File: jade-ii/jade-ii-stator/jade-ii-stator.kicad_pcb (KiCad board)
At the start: 2 copper layers, 93 x 127.3 mm, 0 parts

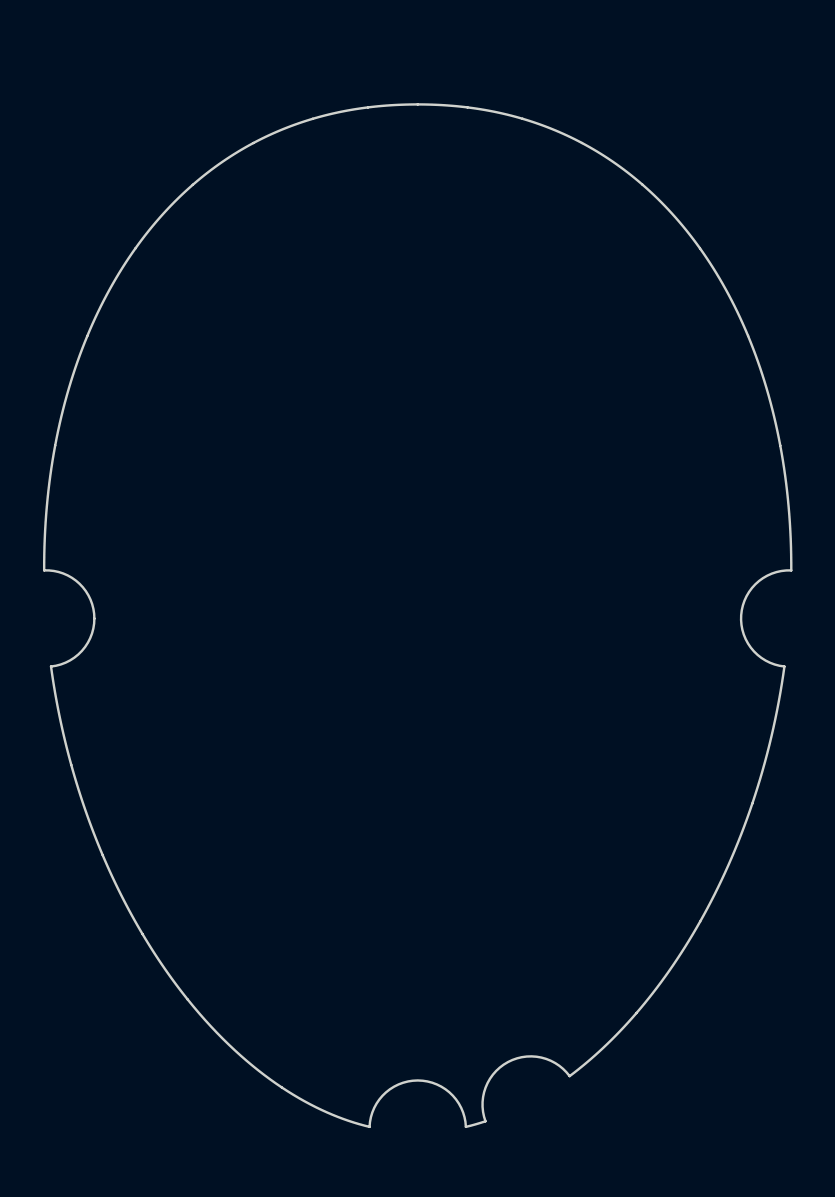
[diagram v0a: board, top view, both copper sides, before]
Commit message: jade: finished stator
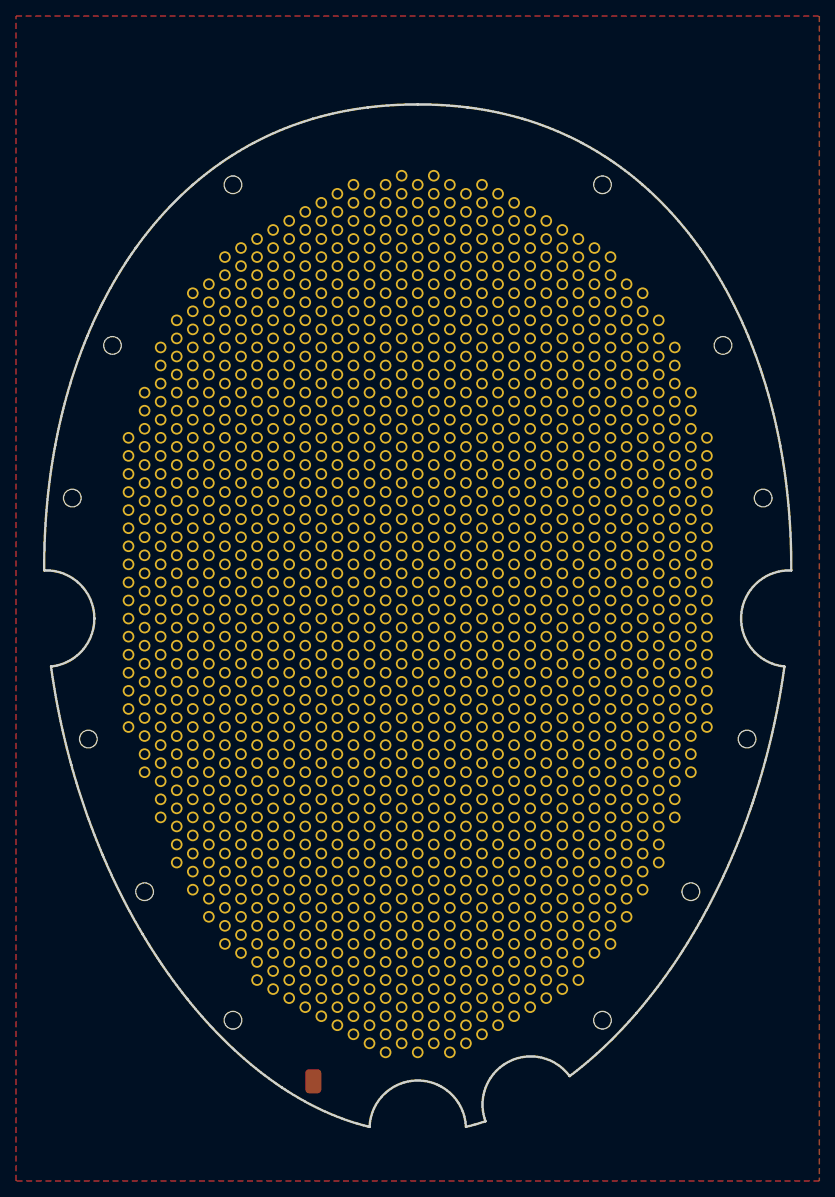
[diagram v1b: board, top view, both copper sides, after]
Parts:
- added H1: MountingHole_Pad, MountingHole:MountingHole_2.2mm_M2_Pad, F.Cu at (26.0, -12.4)
- added H1: MountingHole_Pad, MountingHole:MountingHole_2.2mm_M2_Pad, F.Cu at (-2.00, 12.4)
- added H1: MountingHole_Pad, MountingHole:MountingHole_2.2mm_M2_Pad, F.Cu at (8.00, -31.5)
- added H1: MountingHole_Pad, MountingHole:MountingHole_2.2mm_M2_Pad, F.Cu at (-28.0, 15.8)
- added H1: MountingHole_Pad, MountingHole:MountingHole_2.2mm_M2_Pad, F.Cu at (-10.0, -50.6)
- added H1: MountingHole_Pad, MountingHole:MountingHole_2.2mm_M2_Pad, F.Cu at (-16.0, -24.8)
- added H1: MountingHole_Pad, MountingHole:MountingHole_2.2mm_M2_Pad, F.Cu at (-4.00, 20.2)
- added H1: MountingHole_Pad, MountingHole:MountingHole_2.2mm_M2_Pad, F.Cu at (18.0, -21.4)
- added H1: MountingHole_Pad, MountingHole:MountingHole_2.2mm_M2_Pad, F.Cu at (0.00, 36.0)
- added H1: MountingHole_Pad, MountingHole:MountingHole_2.2mm_M2_Pad, F.Cu at (8.00, 0.00)
- added H1: MountingHole_Pad, MountingHole:MountingHole_2.2mm_M2_Pad, F.Cu at (22.0, 5.62)
- added H1: MountingHole_Pad, MountingHole:MountingHole_2.2mm_M2_Pad, F.Cu at (12.0, -27.0)
- added H1: MountingHole_Pad, MountingHole:MountingHole_2.2mm_M2_Pad, F.Cu at (12.0, -31.5)
- added H1: MountingHole_Pad, MountingHole:MountingHole_2.2mm_M2_Pad, F.Cu at (-4.00, 0.00)
- added H1: MountingHole_Pad, MountingHole:MountingHole_2.2mm_M2_Pad, F.Cu at (-20.0, 9.00)
- added H1: MountingHole_Pad, MountingHole:MountingHole_2.2mm_M2_Pad, F.Cu at (-12.0, 47.2)
- added H1: MountingHole_Pad, MountingHole:MountingHole_2.2mm_M2_Pad, F.Cu at (16.0, -31.5)
- added H1: MountingHole_Pad, MountingHole:MountingHole_2.2mm_M2_Pad, F.Cu at (20.0, -36.0)
- added H1: MountingHole_Pad, MountingHole:MountingHole_2.2mm_M2_Pad, F.Cu at (-2.00, 43.9)
- added H1: MountingHole_Pad, MountingHole:MountingHole_2.2mm_M2_Pad, F.Cu at (4.00, -51.8)
- added H1: MountingHole_Pad, MountingHole:MountingHole_2.2mm_M2_Pad, F.Cu at (26.0, 5.62)
- added H1: MountingHole_Pad, MountingHole:MountingHole_2.2mm_M2_Pad, F.Cu at (-18.0, -1.12)
- added H1: MountingHole_Pad, MountingHole:MountingHole_2.2mm_M2_Pad, F.Cu at (8.00, 49.5)
- added H1: MountingHole_Pad, MountingHole:MountingHole_2.2mm_M2_Pad, F.Cu at (26.0, -41.6)
- added H1: MountingHole_Pad, MountingHole:MountingHole_2.2mm_M2_Pad, F.Cu at (-14.0, 46.1)
- added H1: MountingHole_Pad, MountingHole:MountingHole_2.2mm_M2_Pad, F.Cu at (22.0, 21.4)
- added H1: MountingHole_Pad, MountingHole:MountingHole_2.2mm_M2_Pad, F.Cu at (-16.0, 2.25)
- added H1: MountingHole_Pad, MountingHole:MountingHole_2.2mm_M2_Pad, F.Cu at (26.0, 30.4)
- added H1: MountingHole_Pad, MountingHole:MountingHole_2.2mm_M2_Pad, F.Cu at (-28.0, -33.8)
- added H1: MountingHole_Pad, MountingHole:MountingHole_2.2mm_M2_Pad, F.Cu at (0.00, 51.8)
- added H1: MountingHole_Pad, MountingHole:MountingHole_2.2mm_M2_Pad, F.Cu at (20.0, 18.0)
- added H1: MountingHole_Pad, MountingHole:MountingHole_2.2mm_M2_Pad, F.Cu at (-2.00, 37.1)
- added H1: MountingHole_Pad, MountingHole:MountingHole_2.2mm_M2_Pad, F.Cu at (-10.0, -52.9)
- added H1: MountingHole_Pad, MountingHole:MountingHole_2.2mm_M2_Pad, F.Cu at (-2.00, 41.6)
- added H1: MountingHole_Pad, MountingHole:MountingHole_2.2mm_M2_Pad, F.Cu at (18.0, -10.1)
- added H1: MountingHole_Pad, MountingHole:MountingHole_2.2mm_M2_Pad, F.Cu at (-34.0, 1.12)
- added H1: MountingHole_Pad, MountingHole:MountingHole_2.2mm_M2_Pad, F.Cu at (26.0, 19.1)
- added H1: MountingHole_Pad, MountingHole:MountingHole_2.2mm_M2_Pad, F.Cu at (0.00, 22.5)
- added H1: MountingHole_Pad, MountingHole:MountingHole_2.2mm_M2_Pad, F.Cu at (-18.0, 12.4)
- added H1: MountingHole_Pad, MountingHole:MountingHole_2.2mm_M2_Pad, F.Cu at (-18.0, -21.4)
- added H1: MountingHole_Pad, MountingHole:MountingHole_2.2mm_M2_Pad, F.Cu at (-26.0, 1.12)
- added H1: MountingHole_Pad, MountingHole:MountingHole_2.2mm_M2_Pad, F.Cu at (-2.00, -34.9)
- added H1: MountingHole_Pad, MountingHole:MountingHole_2.2mm_M2_Pad, F.Cu at (14.0, -30.4)
- added H1: MountingHole_Pad, MountingHole:MountingHole_2.2mm_M2_Pad, F.Cu at (-16.0, 22.5)
- added H1: MountingHole_Pad, MountingHole:MountingHole_2.2mm_M2_Pad, F.Cu at (-6.00, 10.1)
- added H1: MountingHole_Pad, MountingHole:MountingHole_2.2mm_M2_Pad, F.Cu at (28.0, 33.8)
- added H1: MountingHole_Pad, MountingHole:MountingHole_2.2mm_M2_Pad, F.Cu at (-32.0, 6.75)
- added H1: MountingHole_Pad, MountingHole:MountingHole_2.2mm_M2_Pad, F.Cu at (-6.00, 19.1)
- added H1: MountingHole_Pad, MountingHole:MountingHole_2.2mm_M2_Pad, F.Cu at (-8.00, -29.2)
- added H1: MountingHole_Pad, MountingHole:MountingHole_2.2mm_M2_Pad, F.Cu at (-18.0, 28.1)
- added H1: MountingHole_Pad, MountingHole:MountingHole_2.2mm_M2_Pad, F.Cu at (30.0, -32.6)
- added H1: MountingHole_Pad, MountingHole:MountingHole_2.2mm_M2_Pad, F.Cu at (0.00, 47.2)
- added H1: MountingHole_Pad, MountingHole:MountingHole_2.2mm_M2_Pad, F.Cu at (8.00, -9.00)
- added H1: MountingHole_Pad, MountingHole:MountingHole_2.2mm_M2_Pad, F.Cu at (6.00, 37.1)
- added H1: MountingHole_Pad, MountingHole:MountingHole_2.2mm_M2_Pad, F.Cu at (-4.00, -20.2)
- added H1: MountingHole_Pad, MountingHole:MountingHole_2.2mm_M2_Pad, F.Cu at (28.0, -20.2)
- added H1: MountingHole_Pad, MountingHole:MountingHole_2.2mm_M2_Pad, F.Cu at (16.0, 42.8)
- added H1: MountingHole_Pad, MountingHole:MountingHole_2.2mm_M2_Pad, F.Cu at (22.0, -5.62)
- added H1: MountingHole_Pad, MountingHole:MountingHole_2.2mm_M2_Pad, F.Cu at (16.0, -13.5)
- added H1: MountingHole_Pad, MountingHole:MountingHole_2.2mm_M2_Pad, F.Cu at (-8.00, 27.0)
- added H1: MountingHole_Pad, MountingHole:MountingHole_2.2mm_M2_Pad, F.Cu at (2.00, 48.4)
- added H1: MountingHole_Pad, MountingHole:MountingHole_2.2mm_M2_Pad, F.Cu at (-22.0, -10.1)
- added H1: MountingHole_Pad, MountingHole:MountingHole_2.2mm_M2_Pad, F.Cu at (4.00, -13.5)
- added H1: MountingHole_Pad, MountingHole:MountingHole_2.2mm_M2_Pad, F.Cu at (4.00, 42.8)
- added H1: MountingHole_Pad, MountingHole:MountingHole_2.2mm_M2_Pad, F.Cu at (20.0, -45.0)
- added H1: MountingHole_Pad, MountingHole:MountingHole_2.2mm_M2_Pad, F.Cu at (-22.0, -34.9)
- added H1: MountingHole_Pad, MountingHole:MountingHole_2.2mm_M2_Pad, F.Cu at (0.00, -33.8)
- added H1: MountingHole_Pad, MountingHole:MountingHole_2.2mm_M2_Pad, F.Cu at (30.0, 7.88)
- added H1: MountingHole_Pad, MountingHole:MountingHole_2.2mm_M2_Pad, F.Cu at (12.0, 40.5)
- added H1: MountingHole_Pad, MountingHole:MountingHole_2.2mm_M2_Pad, F.Cu at (-36.0, 4.50)
- added H1: MountingHole_Pad, MountingHole:MountingHole_2.2mm_M2_Pad, F.Cu at (-2.00, -52.9)
- added H1: MountingHole_Pad, MountingHole:MountingHole_2.2mm_M2_Pad, F.Cu at (4.00, -42.8)
- added H1: MountingHole_Pad, MountingHole:MountingHole_2.2mm_M2_Pad, F.Cu at (-32.0, 11.2)
- added H1: MountingHole_Pad, MountingHole:MountingHole_2.2mm_M2_Pad, F.Cu at (-34.0, 12.4)
- added H1: MountingHole_Pad, MountingHole:MountingHole_2.2mm_M2_Pad, F.Cu at (16.0, 2.25)
- added H1: MountingHole_Pad, MountingHole:MountingHole_2.2mm_M2_Pad, F.Cu at (-22.0, 25.9)
- added H1: MountingHole_Pad, MountingHole:MountingHole_2.2mm_M2_Pad, F.Cu at (22.0, -43.9)
- added H1: MountingHole_Pad, MountingHole:MountingHole_2.2mm_M2_Pad, F.Cu at (28.0, -29.2)
- added H1: MountingHole_Pad, MountingHole:MountingHole_2.2mm_M2_Pad, F.Cu at (-4.00, -6.75)
- added H1: MountingHole_Pad, MountingHole:MountingHole_2.2mm_M2_Pad, F.Cu at (16.0, -45.0)
- added H1: MountingHole_Pad, MountingHole:MountingHole_2.2mm_M2_Pad, F.Cu at (10.0, -5.62)
- added H1: MountingHole_Pad, MountingHole:MountingHole_2.2mm_M2_Pad, F.Cu at (2.00, -10.1)
- added H1: MountingHole_Pad, MountingHole:MountingHole_2.2mm_M2_Pad, F.Cu at (-18.0, 32.6)
- added H1: MountingHole_Pad, MountingHole:MountingHole_2.2mm_M2_Pad, F.Cu at (6.00, -50.6)
- added H1: MountingHole_Pad, MountingHole:MountingHole_2.2mm_M2_Pad, F.Cu at (-32.0, -13.5)
- added H1: MountingHole_Pad, MountingHole:MountingHole_2.2mm_M2_Pad, F.Cu at (-26.0, 30.4)
- added H1: MountingHole_Pad, MountingHole:MountingHole_2.2mm_M2_Pad, F.Cu at (-10.0, 39.4)
- added H1: MountingHole_Pad, MountingHole:MountingHole_2.2mm_M2_Pad, F.Cu at (-36.0, 2.25)
- added H1: MountingHole_Pad, MountingHole:MountingHole_2.2mm_M2_Pad, F.Cu at (6.00, 39.4)
- added H1: MountingHole_Pad, MountingHole:MountingHole_2.2mm_M2_Pad, F.Cu at (-6.00, -16.9)
- added H1: MountingHole_Pad, MountingHole:MountingHole_2.2mm_M2_Pad, F.Cu at (34.0, 5.62)
- added H1: MountingHole_Pad, MountingHole:MountingHole_2.2mm_M2_Pad, F.Cu at (-8.00, -20.2)
- added H1: MountingHole_Pad, MountingHole:MountingHole_2.2mm_M2_Pad, F.Cu at (-12.0, -20.2)
- added H1: MountingHole_Pad, MountingHole:MountingHole_2.2mm_M2_Pad, F.Cu at (-14.0, 16.9)
- added H1: MountingHole_Pad, MountingHole:MountingHole_2.2mm_M2_Pad, F.Cu at (28.0, -36.0)
- added H1: MountingHole_Pad, MountingHole:MountingHole_2.2mm_M2_Pad, F.Cu at (-6.00, -3.38)
- added H1: MountingHole_Pad, MountingHole:MountingHole_2.2mm_M2_Pad, F.Cu at (8.00, 13.5)
- added H1: MountingHole_Pad, MountingHole:MountingHole_2.2mm_M2_Pad, F.Cu at (10.0, 25.9)
- added H1: MountingHole_Pad, MountingHole:MountingHole_2.2mm_M2_Pad, F.Cu at (-2.00, -10.1)
- added H1: MountingHole_Pad, MountingHole:MountingHole_2.2mm_M2_Pad, F.Cu at (22.0, 39.4)
- added H1: MountingHole_Pad, MountingHole:MountingHole_2.2mm_M2_Pad, F.Cu at (14.0, -21.4)
- added H1: MountingHole_Pad, MountingHole:MountingHole_2.2mm_M2_Pad, F.Cu at (-12.0, -29.2)
- added H1: MountingHole_Pad, MountingHole:MountingHole_2.2mm_M2_Pad, F.Cu at (4.00, -2.25)
- added H1: MountingHole_Pad, MountingHole:MountingHole_2.2mm_M2_Pad, F.Cu at (-8.00, -4.50)
- added H1: MountingHole_Pad, MountingHole:MountingHole_2.2mm_M2_Pad, F.Cu at (-8.00, -54.0)
- added H1: MountingHole_Pad, MountingHole:MountingHole_2.2mm_M2_Pad, F.Cu at (4.00, 2.25)
- added H1: MountingHole_Pad, MountingHole:MountingHole_2.2mm_M2_Pad, F.Cu at (32.0, -13.5)
- added H1: MountingHole_Pad, MountingHole:MountingHole_2.2mm_M2_Pad, F.Cu at (14.0, 28.1)
- added H1: MountingHole_Pad, MountingHole:MountingHole_2.2mm_M2_Pad, F.Cu at (2.00, -23.6)
- added H1: MountingHole_Pad, MountingHole:MountingHole_2.2mm_M2_Pad, F.Cu at (-22.0, -32.6)
- added H1: MountingHole_Pad, MountingHole:MountingHole_2.2mm_M2_Pad, F.Cu at (14.0, 30.4)
- added H1: MountingHole_Pad, MountingHole:MountingHole_2.2mm_M2_Pad, F.Cu at (14.0, 7.88)
- added H1: MountingHole_Pad, MountingHole:MountingHole_2.2mm_M2_Pad, F.Cu at (-16.0, -6.75)
- added H1: MountingHole_Pad, MountingHole:MountingHole_2.2mm_M2_Pad, F.Cu at (14.0, 21.4)
- added H1: MountingHole_Pad, MountingHole:MountingHole_2.2mm_M2_Pad, F.Cu at (4.00, 24.8)
- added H1: MountingHole_Pad, MountingHole:MountingHole_2.2mm_M2_Pad, F.Cu at (30.0, -14.6)
- added H1: MountingHole_Pad, MountingHole:MountingHole_2.2mm_M2_Pad, F.Cu at (-4.00, 24.8)
- added H1: MountingHole_Pad, MountingHole:MountingHole_2.2mm_M2_Pad, F.Cu at (14.0, 46.1)
- added H1: MountingHole_Pad, MountingHole:MountingHole_2.2mm_M2_Pad, F.Cu at (-20.0, -2.25)
- added H1: MountingHole_Pad, MountingHole:MountingHole_2.2mm_M2_Pad, F.Cu at (-22.0, 39.4)
- added H1: MountingHole_Pad, MountingHole:MountingHole_2.2mm_M2_Pad, F.Cu at (-10.0, 50.6)
- added H1: MountingHole_Pad, MountingHole:MountingHole_2.2mm_M2_Pad, F.Cu at (0.00, 11.2)
- added H1: MountingHole_Pad, MountingHole:MountingHole_2.2mm_M2_Pad, F.Cu at (28.0, 15.8)
- added H1: MountingHole_Pad, MountingHole:MountingHole_2.2mm_M2_Pad, F.Cu at (-4.00, 4.50)
- added H1: MountingHole_Pad, MountingHole:MountingHole_2.2mm_M2_Pad, F.Cu at (20.0, 38.2)
- added H1: MountingHole_Pad, MountingHole:MountingHole_2.2mm_M2_Pad, F.Cu at (-16.0, -18.0)
- added H1: MountingHole_Pad, MountingHole:MountingHole_2.2mm_M2_Pad, F.Cu at (18.0, -32.6)
- added H1: MountingHole_Pad, MountingHole:MountingHole_2.2mm_M2_Pad, F.Cu at (32.0, -15.8)
- added H1: MountingHole_Pad, MountingHole:MountingHole_2.2mm_M2_Pad, F.Cu at (-20.0, 33.8)
- added H1: MountingHole_Pad, MountingHole:MountingHole_2.2mm_M2_Pad, F.Cu at (20.0, 13.5)
- added H1: MountingHole_Pad, MountingHole:MountingHole_2.2mm_M2_Pad, F.Cu at (34.0, 12.4)
- added H1: MountingHole_Pad, MountingHole:MountingHole_2.2mm_M2_Pad, F.Cu at (20.0, 0.00)
- added H1: MountingHole_Pad, MountingHole:MountingHole_2.2mm_M2_Pad, F.Cu at (-26.0, 5.62)
- added H1: MountingHole_Pad, MountingHole:MountingHole_2.2mm_M2_Pad, F.Cu at (-4.00, -33.8)
- added H1: MountingHole_Pad, MountingHole:MountingHole_2.2mm_M2_Pad, F.Cu at (-4.00, -36.0)
- added H1: MountingHole_Pad, MountingHole:MountingHole_2.2mm_M2_Pad, F.Cu at (22.0, -41.6)
- added H1: MountingHole_Pad, MountingHole:MountingHole_2.2mm_M2_Pad, F.Cu at (26.0, 32.6)
- added H1: MountingHole_Pad, MountingHole:MountingHole_2.2mm_M2_Pad, F.Cu at (-24.0, 11.2)
- added H1: MountingHole_Pad, MountingHole:MountingHole_2.2mm_M2_Pad, F.Cu at (4.00, 13.5)
- added H1: MountingHole_Pad, MountingHole:MountingHole_2.2mm_M2_Pad, F.Cu at (30.0, -5.62)
- added H1: MountingHole_Pad, MountingHole:MountingHole_2.2mm_M2_Pad, F.Cu at (4.00, 22.5)
- added H1: MountingHole_Pad, MountingHole:MountingHole_2.2mm_M2_Pad, F.Cu at (-12.0, -49.5)
- added H1: MountingHole_Pad, MountingHole:MountingHole_2.2mm_M2_Pad, F.Cu at (2.00, -39.4)
- added H1: MountingHole_Pad, MountingHole:MountingHole_2.2mm_M2_Pad, F.Cu at (-6.00, -48.4)
- added H1: MountingHole_Pad, MountingHole:MountingHole_2.2mm_M2_Pad, F.Cu at (-26.0, -3.38)
- added H1: MountingHole_Pad, MountingHole:MountingHole_2.2mm_M2_Pad, F.Cu at (-32.0, -6.75)
- added H1: MountingHole_Pad, MountingHole:MountingHole_2.2mm_M2_Pad, F.Cu at (0.00, 33.8)
- added H1: MountingHole_Pad, MountingHole:MountingHole_2.2mm_M2_Pad, F.Cu at (-4.00, -42.8)
- added H1: MountingHole_Pad, MountingHole:MountingHole_2.2mm_M2_Pad, F.Cu at (12.0, -36.0)
- added H1: MountingHole_Pad, MountingHole:MountingHole_2.2mm_M2_Pad, F.Cu at (-10.0, 23.6)
- added H1: MountingHole_Pad, MountingHole:MountingHole_2.2mm_M2_Pad, F.Cu at (16.0, 33.8)
- added H1: MountingHole_Pad, MountingHole:MountingHole_2.2mm_M2_Pad, F.Cu at (-14.0, -3.38)
- added H1: MountingHole_Pad, MountingHole:MountingHole_2.2mm_M2_Pad, F.Cu at (20.0, 15.8)
- added H1: MountingHole_Pad, MountingHole:MountingHole_2.2mm_M2_Pad, F.Cu at (-18.0, 34.9)
- added H1: MountingHole_Pad, MountingHole:MountingHole_2.2mm_M2_Pad, F.Cu at (-32.0, 2.25)
- added H1: MountingHole_Pad, MountingHole:MountingHole_2.2mm_M2_Pad, F.Cu at (-26.0, -5.62)
- added H1: MountingHole_Pad, MountingHole:MountingHole_2.2mm_M2_Pad, F.Cu at (-10.0, -3.38)
- added H1: MountingHole_Pad, MountingHole:MountingHole_2.2mm_M2_Pad, F.Cu at (-4.00, -9.00)
- added H1: MountingHole_Pad, MountingHole:MountingHole_2.2mm_M2_Pad, F.Cu at (-6.00, 41.6)
- added H1: MountingHole_Pad, MountingHole:MountingHole_2.2mm_M2_Pad, F.Cu at (28.0, 0.00)
- added H1: MountingHole_Pad, MountingHole:MountingHole_2.2mm_M2_Pad, F.Cu at (4.00, 4.50)
- added H1: MountingHole_Pad, MountingHole:MountingHole_2.2mm_M2_Pad, F.Cu at (18.0, -48.4)
- added H1: MountingHole_Pad, MountingHole:MountingHole_2.2mm_M2_Pad, F.Cu at (-20.0, -11.2)
- added H1: MountingHole_Pad, MountingHole:MountingHole_2.2mm_M2_Pad, F.Cu at (-32.0, 4.50)
- added H1: MountingHole_Pad, MountingHole:MountingHole_2.2mm_M2_Pad, F.Cu at (-16.0, -13.5)
- added H1: MountingHole_Pad, MountingHole:MountingHole_2.2mm_M2_Pad, F.Cu at (10.0, 50.6)
- added H1: MountingHole_Pad, MountingHole:MountingHole_2.2mm_M2_Pad, F.Cu at (2.00, 39.4)
- added H1: MountingHole_Pad, MountingHole:MountingHole_2.2mm_M2_Pad, F.Cu at (6.00, -5.62)
- added H1: MountingHole_Pad, MountingHole:MountingHole_2.2mm_M2_Pad, F.Cu at (-8.00, -40.5)
- added H1: MountingHole_Pad, MountingHole:MountingHole_2.2mm_M2_Pad, F.Cu at (-26.0, -34.9)
- added H1: MountingHole_Pad, MountingHole:MountingHole_2.2mm_M2_Pad, F.Cu at (-28.0, 29.2)
- added H1: MountingHole_Pad, MountingHole:MountingHole_2.2mm_M2_Pad, F.Cu at (-14.0, -25.9)
- added H1: MountingHole_Pad, MountingHole:MountingHole_2.2mm_M2_Pad, F.Cu at (14.0, -19.1)
- added H1: MountingHole_Pad, MountingHole:MountingHole_2.2mm_M2_Pad, F.Cu at (-16.0, -20.2)
- added H1: MountingHole_Pad, MountingHole:MountingHole_2.2mm_M2_Pad, F.Cu at (22.0, -12.4)
- added H1: MountingHole_Pad, MountingHole:MountingHole_2.2mm_M2_Pad, F.Cu at (22.0, 3.38)
- added H1: MountingHole_Pad, MountingHole:MountingHole_2.2mm_M2_Pad, F.Cu at (-4.00, 40.5)
- added H1: MountingHole_Pad, MountingHole:MountingHole_2.2mm_M2_Pad, F.Cu at (20.0, -47.2)
- added H1: MountingHole_Pad, MountingHole:MountingHole_2.2mm_M2_Pad, F.Cu at (18.0, -41.6)
- added H1: MountingHole_Pad, MountingHole:MountingHole_2.2mm_M2_Pad, F.Cu at (24.0, 38.2)
- added H1: MountingHole_Pad, MountingHole:MountingHole_2.2mm_M2_Pad, F.Cu at (22.0, -1.12)
- added H1: MountingHole_Pad, MountingHole:MountingHole_2.2mm_M2_Pad, F.Cu at (-4.00, 9.00)
- added H1: MountingHole_Pad, MountingHole:MountingHole_2.2mm_M2_Pad, F.Cu at (8.00, 45.0)
- added H1: MountingHole_Pad, MountingHole:MountingHole_2.2mm_M2_Pad, F.Cu at (-12.0, -42.8)
- added H1: MountingHole_Pad, MountingHole:MountingHole_2.2mm_M2_Pad, F.Cu at (-10.0, 25.9)
- added H1: MountingHole_Pad, MountingHole:MountingHole_2.2mm_M2_Pad, F.Cu at (-12.0, 22.5)
- added H1: MountingHole_Pad, MountingHole:MountingHole_2.2mm_M2_Pad, F.Cu at (-4.00, -54.0)
- added H1: MountingHole_Pad, MountingHole:MountingHole_2.2mm_M2_Pad, F.Cu at (16.0, 45.0)
- added H1: MountingHole_Pad, MountingHole:MountingHole_2.2mm_M2_Pad, F.Cu at (24.0, -6.75)
- added H1: MountingHole_Pad, MountingHole:MountingHole_2.2mm_M2_Pad, F.Cu at (-2.00, -1.12)
- added H1: MountingHole_Pad, MountingHole:MountingHole_2.2mm_M2_Pad, F.Cu at (8.00, 42.8)
- added H1: MountingHole_Pad, MountingHole:MountingHole_2.2mm_M2_Pad, F.Cu at (14.0, -46.1)
- added H1: MountingHole_Pad, MountingHole:MountingHole_2.2mm_M2_Pad, F.Cu at (-20.0, -36.0)
- added H1: MountingHole_Pad, MountingHole:MountingHole_2.2mm_M2_Pad, F.Cu at (30.0, -12.4)
- added H1: MountingHole_Pad, MountingHole:MountingHole_2.2mm_M2_Pad, F.Cu at (-20.0, 2.25)
- added H1: MountingHole_Pad, MountingHole:MountingHole_2.2mm_M2_Pad, F.Cu at (20.0, 2.25)
- added H1: MountingHole_Pad, MountingHole:MountingHole_2.2mm_M2_Pad, F.Cu at (-18.0, 43.9)
- added H1: MountingHole_Pad, MountingHole:MountingHole_2.2mm_M2_Pad, F.Cu at (-24.0, 20.2)
- added H1: MountingHole_Pad, MountingHole:MountingHole_2.2mm_M2_Pad, F.Cu at (-14.0, -48.4)
- added H1: MountingHole_Pad, MountingHole:MountingHole_2.2mm_M2_Pad, F.Cu at (-22.0, -16.9)
- added H1: MountingHole_Pad, MountingHole:MountingHole_2.2mm_M2_Pad, F.Cu at (-6.00, -23.6)
- added H1: MountingHole_Pad, MountingHole:MountingHole_2.2mm_M2_Pad, F.Cu at (-24.0, -45.0)
- added H1: MountingHole_Pad, MountingHole:MountingHole_2.2mm_M2_Pad, F.Cu at (14.0, -48.4)
- added H1: MountingHole_Pad, MountingHole:MountingHole_2.2mm_M2_Pad, F.Cu at (-10.0, 28.1)
- added H1: MountingHole_Pad, MountingHole:MountingHole_2.2mm_M2_Pad, F.Cu at (24.0, 31.5)
- added H1: MountingHole_Pad, MountingHole:MountingHole_2.2mm_M2_Pad, F.Cu at (6.00, -1.12)
- added H1: MountingHole_Pad, MountingHole:MountingHole_2.2mm_M2_Pad, F.Cu at (-36.0, -15.8)
- added H1: MountingHole_Pad, MountingHole:MountingHole_2.2mm_M2_Pad, F.Cu at (18.0, -28.1)
- added H1: MountingHole_Pad, MountingHole:MountingHole_2.2mm_M2_Pad, F.Cu at (24.0, -31.5)
- added H1: MountingHole_Pad, MountingHole:MountingHole_2.2mm_M2_Pad, F.Cu at (-6.00, -37.1)
- added H1: MountingHole_Pad, MountingHole:MountingHole_2.2mm_M2_Pad, F.Cu at (-24.0, -22.5)
- added H1: MountingHole_Pad, MountingHole:MountingHole_2.2mm_M2_Pad, F.Cu at (28.0, -15.8)
- added H1: MountingHole_Pad, MountingHole:MountingHole_2.2mm_M2_Pad, F.Cu at (-28.0, -31.5)
- added H1: MountingHole_Pad, MountingHole:MountingHole_2.2mm_M2_Pad, F.Cu at (-2.00, 1.12)
- added H1: MountingHole_Pad, MountingHole:MountingHole_2.2mm_M2_Pad, F.Cu at (10.0, -50.6)
- added H1: MountingHole_Pad, MountingHole:MountingHole_2.2mm_M2_Pad, F.Cu at (4.00, -24.8)
- added H1: MountingHole_Pad, MountingHole:MountingHole_2.2mm_M2_Pad, F.Cu at (-18.0, -32.6)
- added H1: MountingHole_Pad, MountingHole:MountingHole_2.2mm_M2_Pad, F.Cu at (30.0, 3.38)
- added H1: MountingHole_Pad, MountingHole:MountingHole_2.2mm_M2_Pad, F.Cu at (-30.0, -5.62)
- added H1: MountingHole_Pad, MountingHole:MountingHole_2.2mm_M2_Pad, F.Cu at (32.0, -24.8)
- added H1: MountingHole_Pad, MountingHole:MountingHole_2.2mm_M2_Pad, F.Cu at (32.0, 11.2)
- added H1: MountingHole_Pad, MountingHole:MountingHole_2.2mm_M2_Pad, F.Cu at (16.0, 24.8)
- added H1: MountingHole_Pad, MountingHole:MountingHole_2.2mm_M2_Pad, F.Cu at (-26.0, -12.4)
- added H1: MountingHole_Pad, MountingHole:MountingHole_2.2mm_M2_Pad, F.Cu at (-16.0, 24.8)
- added H1: MountingHole_Pad, MountingHole:MountingHole_2.2mm_M2_Pad, F.Cu at (6.00, 46.1)
- added H1: MountingHole_Pad, MountingHole:MountingHole_2.2mm_M2_Pad, F.Cu at (16.0, -22.5)
- added H1: MountingHole_Pad, MountingHole:MountingHole_2.2mm_M2_Pad, F.Cu at (6.00, -28.1)
- added H1: MountingHole_Pad, MountingHole:MountingHole_2.2mm_M2_Pad, F.Cu at (-16.0, -36.0)
- added H1: MountingHole_Pad, MountingHole:MountingHole_2.2mm_M2_Pad, F.Cu at (12.0, 27.0)
- added H1: MountingHole_Pad, MountingHole:MountingHole_2.2mm_M2_Pad, F.Cu at (18.0, 16.9)
- added H1: MountingHole_Pad, MountingHole:MountingHole_2.2mm_M2_Pad, F.Cu at (-16.0, -49.5)
- added H1: MountingHole_Pad, MountingHole:MountingHole_2.2mm_M2_Pad, F.Cu at (32.0, -11.2)
- added H1: MountingHole_Pad, MountingHole:MountingHole_2.2mm_M2_Pad, F.Cu at (4.00, -20.2)
- added H1: MountingHole_Pad, MountingHole:MountingHole_2.2mm_M2_Pad, F.Cu at (26.0, -7.88)
- added H1: MountingHole_Pad, MountingHole:MountingHole_2.2mm_M2_Pad, F.Cu at (24.0, 27.0)
- added H1: MountingHole_Pad, MountingHole:MountingHole_2.2mm_M2_Pad, F.Cu at (8.00, -27.0)
- added H1: MountingHole_Pad, MountingHole:MountingHole_2.2mm_M2_Pad, F.Cu at (-6.00, 28.1)
- added H1: MountingHole_Pad, MountingHole:MountingHole_2.2mm_M2_Pad, F.Cu at (28.0, 13.5)
- added H1: MountingHole_Pad, MountingHole:MountingHole_2.2mm_M2_Pad, F.Cu at (8.00, 36.0)
- added H1: MountingHole_Pad, MountingHole:MountingHole_2.2mm_M2_Pad, F.Cu at (-14.0, 21.4)
- added H1: MountingHole_Pad, MountingHole:MountingHole_2.2mm_M2_Pad, F.Cu at (-26.0, -7.88)
- added H1: MountingHole_Pad, MountingHole:MountingHole_2.2mm_M2_Pad, F.Cu at (12.0, -51.8)
- added H1: MountingHole_Pad, MountingHole:MountingHole_2.2mm_M2_Pad, F.Cu at (14.0, 16.9)
- added H1: MountingHole_Pad, MountingHole:MountingHole_2.2mm_M2_Pad, F.Cu at (-2.00, 7.88)
- added H1: MountingHole_Pad, MountingHole:MountingHole_2.2mm_M2_Pad, F.Cu at (2.00, 5.62)
- added H1: MountingHole_Pad, MountingHole:MountingHole_2.2mm_M2_Pad, F.Cu at (-12.0, -13.5)
- added H1: MountingHole_Pad, MountingHole:MountingHole_2.2mm_M2_Pad, F.Cu at (30.0, 16.9)
- added H1: MountingHole_Pad, MountingHole:MountingHole_2.2mm_M2_Pad, F.Cu at (-30.0, -34.9)
- added H1: MountingHole_Pad, MountingHole:MountingHole_2.2mm_M2_Pad, F.Cu at (10.0, -52.9)
- added H1: MountingHole_Pad, MountingHole:MountingHole_2.2mm_M2_Pad, F.Cu at (34.0, -28.1)
- added H1: MountingHole_Pad, MountingHole:MountingHole_2.2mm_M2_Pad, F.Cu at (-10.0, 46.1)
- added H1: MountingHole_Pad, MountingHole:MountingHole_2.2mm_M2_Pad, F.Cu at (20.0, -9.00)
- added H1: MountingHole_Pad, MountingHole:MountingHole_2.2mm_M2_Pad, F.Cu at (-10.0, 21.4)
- added H1: MountingHole_Pad, MountingHole:MountingHole_2.2mm_M2_Pad, F.Cu at (-22.0, -21.4)
- added H1: MountingHole_Pad, MountingHole:MountingHole_2.2mm_M2_Pad, F.Cu at (10.0, -30.4)
- added H1: MountingHole_Pad, MountingHole:MountingHole_2.2mm_M2_Pad, F.Cu at (18.0, 23.6)
- added H1: MountingHole_Pad, MountingHole:MountingHole_2.2mm_M2_Pad, F.Cu at (-24.0, 29.2)
- added H1: MountingHole_Pad, MountingHole:MountingHole_2.2mm_M2_Pad, F.Cu at (-20.0, -47.2)
- added H1: MountingHole_Pad, MountingHole:MountingHole_2.2mm_M2_Pad, F.Cu at (-16.0, -2.25)
- added H1: MountingHole_Pad, MountingHole:MountingHole_2.2mm_M2_Pad, F.Cu at (-8.00, 49.5)
- added H1: MountingHole_Pad, MountingHole:MountingHole_2.2mm_M2_Pad, F.Cu at (-24.0, -6.75)
- added H1: MountingHole_Pad, MountingHole:MountingHole_2.2mm_M2_Pad, F.Cu at (20.0, 24.8)
- added H1: MountingHole_Pad, MountingHole:MountingHole_2.2mm_M2_Pad, F.Cu at (2.00, 3.38)
- added H1: MountingHole_Pad, MountingHole:MountingHole_2.2mm_M2_Pad, F.Cu at (-6.00, 39.4)
- added H1: MountingHole_Pad, MountingHole:MountingHole_2.2mm_M2_Pad, F.Cu at (2.00, -34.9)
- added H1: MountingHole_Pad, MountingHole:MountingHole_2.2mm_M2_Pad, F.Cu at (-8.00, -38.2)
- added H1: MountingHole_Pad, MountingHole:MountingHole_2.2mm_M2_Pad, F.Cu at (12.0, 11.2)
- added H1: MountingHole_Pad, MountingHole:MountingHole_2.2mm_M2_Pad, F.Cu at (-26.0, 3.38)
- added H1: MountingHole_Pad, MountingHole:MountingHole_2.2mm_M2_Pad, F.Cu at (22.0, 37.1)
- added H1: MountingHole_Pad, MountingHole:MountingHole_2.2mm_M2_Pad, F.Cu at (-18.0, -41.6)
- added H1: MountingHole_Pad, MountingHole:MountingHole_2.2mm_M2_Pad, F.Cu at (-16.0, -27.0)
- added H1: MountingHole_Pad, MountingHole:MountingHole_2.2mm_M2_Pad, F.Cu at (26.0, -25.9)
- added H1: MountingHole_Pad, MountingHole:MountingHole_2.2mm_M2_Pad, F.Cu at (-30.0, -1.12)
- added H1: MountingHole_Pad, MountingHole:MountingHole_2.2mm_M2_Pad, F.Cu at (-28.0, 22.5)
- added H1: MountingHole_Pad, MountingHole:MountingHole_2.2mm_M2_Pad, F.Cu at (8.00, -29.2)
- added H1: MountingHole_Pad, MountingHole:MountingHole_2.2mm_M2_Pad, F.Cu at (32.0, 13.5)
- added H1: MountingHole_Pad, MountingHole:MountingHole_2.2mm_M2_Pad, F.Cu at (-12.0, -6.75)
- added H1: MountingHole_Pad, MountingHole:MountingHole_2.2mm_M2_Pad, F.Cu at (14.0, 14.6)
- added H1: MountingHole_Pad, MountingHole:MountingHole_2.2mm_M2_Pad, F.Cu at (18.0, -43.9)
- added H1: MountingHole_Pad, MountingHole:MountingHole_2.2mm_M2_Pad, F.Cu at (-30.0, -21.4)
- added H1: MountingHole_Pad, MountingHole:MountingHole_2.2mm_M2_Pad, F.Cu at (-28.0, 6.75)
- added H1: MountingHole_Pad, MountingHole:MountingHole_2.2mm_M2_Pad, F.Cu at (4.00, 47.2)
- added H1: MountingHole_Pad, MountingHole:MountingHole_2.2mm_M2_Pad, F.Cu at (18.0, -7.88)
- added H1: MountingHole_Pad, MountingHole:MountingHole_2.2mm_M2_Pad, F.Cu at (-34.0, 5.62)
- added H1: MountingHole_Pad, MountingHole:MountingHole_2.2mm_M2_Pad, F.Cu at (2.00, -7.88)
- added H1: MountingHole_Pad, MountingHole:MountingHole_2.2mm_M2_Pad, F.Cu at (-18.0, 1.12)
- added H1: MountingHole_Pad, MountingHole:MountingHole_2.2mm_M2_Pad, F.Cu at (-26.0, -28.1)
- added H1: MountingHole_Pad, MountingHole:MountingHole_2.2mm_M2_Pad, F.Cu at (22.0, 41.6)
- added H1: MountingHole_Pad, MountingHole:MountingHole_2.2mm_M2_Pad, F.Cu at (-22.0, 21.4)
- added H1: MountingHole_Pad, MountingHole:MountingHole_2.2mm_M2_Pad, F.Cu at (-16.0, 0.00)
- added H1: MountingHole_Pad, MountingHole:MountingHole_2.2mm_M2_Pad, F.Cu at (0.00, 29.2)
- added H1: MountingHole_Pad, MountingHole:MountingHole_2.2mm_M2_Pad, F.Cu at (34.0, 7.88)
- added H1: MountingHole_Pad, MountingHole:MountingHole_2.2mm_M2_Pad, F.Cu at (-36.0, -20.2)
- added H1: MountingHole_Pad, MountingHole:MountingHole_2.2mm_M2_Pad, F.Cu at (-8.00, 36.0)
- added H1: MountingHole_Pad, MountingHole:MountingHole_2.2mm_M2_Pad, F.Cu at (26.0, 3.38)
- added H1: MountingHole_Pad, MountingHole:MountingHole_2.2mm_M2_Pad, F.Cu at (34.0, -10.1)
- added H1: MountingHole_Pad, MountingHole:MountingHole_2.2mm_M2_Pad, F.Cu at (12.0, 38.2)
- added H1: MountingHole_Pad, MountingHole:MountingHole_2.2mm_M2_Pad, F.Cu at (10.0, 46.1)
- added H1: MountingHole_Pad, MountingHole:MountingHole_2.2mm_M2_Pad, F.Cu at (10.0, -16.9)
- added H1: MountingHole_Pad, MountingHole:MountingHole_2.2mm_M2_Pad, F.Cu at (-18.0, 7.88)
- added H1: MountingHole_Pad, MountingHole:MountingHole_2.2mm_M2_Pad, F.Cu at (12.0, 2.25)
- added H1: MountingHole_Pad, MountingHole:MountingHole_2.2mm_M2_Pad, F.Cu at (6.00, 12.4)
- added H1: MountingHole_Pad, MountingHole:MountingHole_2.2mm_M2_Pad, F.Cu at (12.0, -49.5)
- added H1: MountingHole_Pad, MountingHole:MountingHole_2.2mm_M2_Pad, F.Cu at (-14.0, 1.12)
- added H1: MountingHole_Pad, MountingHole:MountingHole_2.2mm_M2_Pad, F.Cu at (-12.0, -24.8)
- added H1: MountingHole_Pad, MountingHole:MountingHole_2.2mm_M2_Pad, F.Cu at (18.0, 12.4)
- added H1: MountingHole_Pad, MountingHole:MountingHole_2.2mm_M2_Pad, F.Cu at (-22.0, -41.6)
- added H1: MountingHole_Pad, MountingHole:MountingHole_2.2mm_M2_Pad, F.Cu at (-36.0, -2.25)
- added H1: MountingHole_Pad, MountingHole:MountingHole_2.2mm_M2_Pad, F.Cu at (0.00, -45.0)
- added H1: MountingHole_Pad, MountingHole:MountingHole_2.2mm_M2_Pad, F.Cu at (-26.0, -41.6)
- added H1: MountingHole_Pad, MountingHole:MountingHole_2.2mm_M2_Pad, F.Cu at (-14.0, -21.4)
- added H1: MountingHole_Pad, MountingHole:MountingHole_2.2mm_M2_Pad, F.Cu at (18.0, -34.9)
- added H1: MountingHole_Pad, MountingHole:MountingHole_2.2mm_M2_Pad, F.Cu at (-10.0, -23.6)
- added H1: MountingHole_Pad, MountingHole:MountingHole_2.2mm_M2_Pad, F.Cu at (-10.0, 41.6)
- added H1: MountingHole_Pad, MountingHole:MountingHole_2.2mm_M2_Pad, F.Cu at (14.0, 37.1)
- added H1: MountingHole_Pad, MountingHole:MountingHole_2.2mm_M2_Pad, F.Cu at (12.0, -42.8)
- added H1: MountingHole_Pad, MountingHole:MountingHole_2.2mm_M2_Pad, F.Cu at (-30.0, 10.1)
- added H1: MountingHole_Pad, MountingHole:MountingHole_2.2mm_M2_Pad, F.Cu at (-6.00, 5.62)
- added H1: MountingHole_Pad, MountingHole:MountingHole_2.2mm_M2_Pad, F.Cu at (-4.00, 11.2)
- added H1: MountingHole_Pad, MountingHole:MountingHole_2.2mm_M2_Pad, F.Cu at (-24.0, 6.75)
- added H1: MountingHole_Pad, MountingHole:MountingHole_2.2mm_M2_Pad, F.Cu at (24.0, -27.0)
- added H1: MountingHole_Pad, MountingHole:MountingHole_2.2mm_M2_Pad, F.Cu at (6.00, 34.9)
- added H1: MountingHole_Pad, MountingHole:MountingHole_2.2mm_M2_Pad, F.Cu at (2.00, -19.1)
- added H1: MountingHole_Pad, MountingHole:MountingHole_2.2mm_M2_Pad, F.Cu at (-26.0, 37.1)
- added H1: MountingHole_Pad, MountingHole:MountingHole_2.2mm_M2_Pad, F.Cu at (28.0, 24.8)
- added H1: MountingHole_Pad, MountingHole:MountingHole_2.2mm_M2_Pad, F.Cu at (-32.0, -24.8)
- added H1: MountingHole_Pad, MountingHole:MountingHole_2.2mm_M2_Pad, F.Cu at (-6.00, -43.9)
- added H1: MountingHole_Pad, MountingHole:MountingHole_2.2mm_M2_Pad, F.Cu at (-18.0, 10.1)
- added H1: MountingHole_Pad, MountingHole:MountingHole_2.2mm_M2_Pad, F.Cu at (-2.00, 14.6)
- added H1: MountingHole_Pad, MountingHole:MountingHole_2.2mm_M2_Pad, F.Cu at (-22.0, 16.9)
- added H1: MountingHole_Pad, MountingHole:MountingHole_2.2mm_M2_Pad, F.Cu at (-6.00, 25.9)
- added H1: MountingHole_Pad, MountingHole:MountingHole_2.2mm_M2_Pad, F.Cu at (-16.0, 31.5)
- added H1: MountingHole_Pad, MountingHole:MountingHole_2.2mm_M2_Pad, F.Cu at (-36.0, -22.5)
- added H1: MountingHole_Pad, MountingHole:MountingHole_2.2mm_M2_Pad, F.Cu at (12.0, 31.5)
- added H1: MountingHole_Pad, MountingHole:MountingHole_2.2mm_M2_Pad, F.Cu at (-10.0, -34.9)
- added H1: MountingHole_Pad, MountingHole:MountingHole_2.2mm_M2_Pad, F.Cu at (36.0, -2.25)
- added H1: MountingHole_Pad, MountingHole:MountingHole_2.2mm_M2_Pad, F.Cu at (-10.0, 10.1)
- added H1: MountingHole_Pad, MountingHole:MountingHole_2.2mm_M2_Pad, F.Cu at (10.0, -3.38)
- added H1: MountingHole_Pad, MountingHole:MountingHole_2.2mm_M2_Pad, F.Cu at (-20.0, 0.00)
- added H1: MountingHole_Pad, MountingHole:MountingHole_2.2mm_M2_Pad, F.Cu at (-14.0, -43.9)
- added H1: MountingHole_Pad, MountingHole:MountingHole_2.2mm_M2_Pad, F.Cu at (-24.0, 4.50)
- added H1: MountingHole_Pad, MountingHole:MountingHole_2.2mm_M2_Pad, F.Cu at (-8.00, 11.2)
- added H1: MountingHole_Pad, MountingHole:MountingHole_2.2mm_M2_Pad, F.Cu at (30.0, 5.62)
- added H1: MountingHole_Pad, MountingHole:MountingHole_2.2mm_M2_Pad, F.Cu at (-8.00, -18.0)
- added H1: MountingHole_Pad, MountingHole:MountingHole_2.2mm_M2_Pad, F.Cu at (6.00, -7.88)
- added H1: MountingHole_Pad, MountingHole:MountingHole_2.2mm_M2_Pad, F.Cu at (34.0, 3.38)
- added H1: MountingHole_Pad, MountingHole:MountingHole_2.2mm_M2_Pad, F.Cu at (-2.00, -16.9)
- added H1: MountingHole_Pad, MountingHole:MountingHole_2.2mm_M2_Pad, F.Cu at (2.00, -21.4)
- added H1: MountingHole_Pad, MountingHole:MountingHole_2.2mm_M2_Pad, F.Cu at (-20.0, -42.8)
- added H1: MountingHole_Pad, MountingHole:MountingHole_2.2mm_M2_Pad, F.Cu at (14.0, -7.88)
- added H1: MountingHole_Pad, MountingHole:MountingHole_2.2mm_M2_Pad, F.Cu at (14.0, 12.4)
- added H1: MountingHole_Pad, MountingHole:MountingHole_2.2mm_M2_Pad, F.Cu at (-4.00, 29.2)
- added H1: MountingHole_Pad, MountingHole:MountingHole_2.2mm_M2_Pad, F.Cu at (-18.0, 41.6)
- added H1: MountingHole_Pad, MountingHole:MountingHole_2.2mm_M2_Pad, F.Cu at (-14.0, -5.62)
- added H1: MountingHole_Pad, MountingHole:MountingHole_2.2mm_M2_Pad, F.Cu at (0.00, -47.2)
- added H1: MountingHole_Pad, MountingHole:MountingHole_2.2mm_M2_Pad, F.Cu at (-22.0, -25.9)
- added H1: MountingHole_Pad, MountingHole:MountingHole_2.2mm_M2_Pad, F.Cu at (-18.0, -5.62)
- added H1: MountingHole_Pad, MountingHole:MountingHole_2.2mm_M2_Pad, F.Cu at (8.00, -18.0)
- added H1: MountingHole_Pad, MountingHole:MountingHole_2.2mm_M2_Pad, F.Cu at (12.0, -45.0)
- added H1: MountingHole_Pad, MountingHole:MountingHole_2.2mm_M2_Pad, F.Cu at (-36.0, 6.75)
- added H1: MountingHole_Pad, MountingHole:MountingHole_2.2mm_M2_Pad, F.Cu at (-16.0, -38.2)
- added H1: MountingHole_Pad, MountingHole:MountingHole_2.2mm_M2_Pad, F.Cu at (10.0, 7.88)
- added H1: MountingHole_Pad, MountingHole:MountingHole_2.2mm_M2_Pad, F.Cu at (6.00, 25.9)
- added H1: MountingHole_Pad, MountingHole:MountingHole_2.2mm_M2_Pad, F.Cu at (6.00, 5.62)
- added H1: MountingHole_Pad, MountingHole:MountingHole_2.2mm_M2_Pad, F.Cu at (10.0, 23.6)
- added H1: MountingHole_Pad, MountingHole:MountingHole_2.2mm_M2_Pad, F.Cu at (-22.0, 37.1)
- added H1: MountingHole_Pad, MountingHole:MountingHole_2.2mm_M2_Pad, F.Cu at (12.0, -11.2)
- added H1: MountingHole_Pad, MountingHole:MountingHole_2.2mm_M2_Pad, F.Cu at (26.0, 34.9)
- added H1: MountingHole_Pad, MountingHole:MountingHole_2.2mm_M2_Pad, F.Cu at (-20.0, -29.2)
- added H1: MountingHole_Pad, MountingHole:MountingHole_2.2mm_M2_Pad, F.Cu at (2.00, -3.38)
- added H1: MountingHole_Pad, MountingHole:MountingHole_2.2mm_M2_Pad, F.Cu at (4.00, -15.8)
- added H1: MountingHole_Pad, MountingHole:MountingHole_2.2mm_M2_Pad, F.Cu at (-26.0, 32.6)
- added H1: MountingHole_Pad, MountingHole:MountingHole_2.2mm_M2_Pad, F.Cu at (10.0, -37.1)
- added H1: MountingHole_Pad, MountingHole:MountingHole_2.2mm_M2_Pad, F.Cu at (6.00, -12.4)
- added H1: MountingHole_Pad, MountingHole:MountingHole_2.2mm_M2_Pad, F.Cu at (-4.00, 2.25)
- added H1: MountingHole_Pad, MountingHole:MountingHole_2.2mm_M2_Pad, F.Cu at (8.00, -47.2)
- added H1: MountingHole_Pad, MountingHole:MountingHole_2.2mm_M2_Pad, F.Cu at (-6.00, 23.6)
- added H1: MountingHole_Pad, MountingHole:MountingHole_2.2mm_M2_Pad, F.Cu at (-24.0, -15.8)
- added H1: MountingHole_Pad, MountingHole:MountingHole_2.2mm_M2_Pad, F.Cu at (20.0, -31.5)
- added H1: MountingHole_Pad, MountingHole:MountingHole_2.2mm_M2_Pad, F.Cu at (10.0, -25.9)
- added H1: MountingHole_Pad, MountingHole:MountingHole_2.2mm_M2_Pad, F.Cu at (-32.0, 18.0)
- added H1: MountingHole_Pad, MountingHole:MountingHole_2.2mm_M2_Pad, F.Cu at (4.00, 36.0)
- added H1: MountingHole_Pad, MountingHole:MountingHole_2.2mm_M2_Pad, F.Cu at (14.0, -34.9)
- added H1: MountingHole_Pad, MountingHole:MountingHole_2.2mm_M2_Pad, F.Cu at (8.00, 22.5)
- added H1: MountingHole_Pad, MountingHole:MountingHole_2.2mm_M2_Pad, F.Cu at (-10.0, -43.9)
- added H1: MountingHole_Pad, MountingHole:MountingHole_2.2mm_M2_Pad, F.Cu at (-12.0, -11.2)
- added H1: MountingHole_Pad, MountingHole:MountingHole_2.2mm_M2_Pad, F.Cu at (-6.00, 14.6)
- added H1: MountingHole_Pad, MountingHole:MountingHole_2.2mm_M2_Pad, F.Cu at (0.00, -24.8)
- added H1: MountingHole_Pad, MountingHole:MountingHole_2.2mm_M2_Pad, F.Cu at (-4.00, -31.5)
- added H1: MountingHole_Pad, MountingHole:MountingHole_2.2mm_M2_Pad, F.Cu at (-6.00, 32.6)
- added H1: MountingHole_Pad, MountingHole:MountingHole_2.2mm_M2_Pad, F.Cu at (-2.00, 32.6)
- added H1: MountingHole_Pad, MountingHole:MountingHole_2.2mm_M2_Pad, F.Cu at (-26.0, -1.12)
- added H1: MountingHole_Pad, MountingHole:MountingHole_2.2mm_M2_Pad, F.Cu at (-2.00, -48.4)
- added H1: MountingHole_Pad, MountingHole:MountingHole_2.2mm_M2_Pad, F.Cu at (-30.0, -3.38)
- added H1: MountingHole_Pad, MountingHole:MountingHole_2.2mm_M2_Pad, F.Cu at (8.00, -45.0)
- added H1: MountingHole_Pad, MountingHole:MountingHole_2.2mm_M2_Pad, F.Cu at (-34.0, 3.38)
- added H1: MountingHole_Pad, MountingHole:MountingHole_2.2mm_M2_Pad, F.Cu at (-6.00, 21.4)
- added H1: MountingHole_Pad, MountingHole:MountingHole_2.2mm_M2_Pad, F.Cu at (16.0, 29.2)
- added H1: MountingHole_Pad, MountingHole:MountingHole_2.2mm_M2_Pad, F.Cu at (-6.00, 12.4)
- added H1: MountingHole_Pad, MountingHole:MountingHole_2.2mm_M2_Pad, F.Cu at (-8.00, 42.8)
- added H1: MountingHole_Pad, MountingHole:MountingHole_2.2mm_M2_Pad, F.Cu at (30.0, -7.88)
- added H1: MountingHole_Pad, MountingHole:MountingHole_2.2mm_M2_Pad, F.Cu at (-32.0, 0.00)
- added H1: MountingHole_Pad, MountingHole:MountingHole_2.2mm_M2_Pad, F.Cu at (-30.0, -37.1)
- added H1: MountingHole_Pad, MountingHole:MountingHole_2.2mm_M2_Pad, F.Cu at (6.00, -37.1)
- added H1: MountingHole_Pad, MountingHole:MountingHole_2.2mm_M2_Pad, F.Cu at (-12.0, 33.8)
- added H1: MountingHole_Pad, MountingHole:MountingHole_2.2mm_M2_Pad, F.Cu at (10.0, 5.62)
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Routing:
- added copper zone on F.Cu, net /Conn
